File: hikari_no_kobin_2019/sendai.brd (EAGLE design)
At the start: 43 x 43 mm, 4 parts

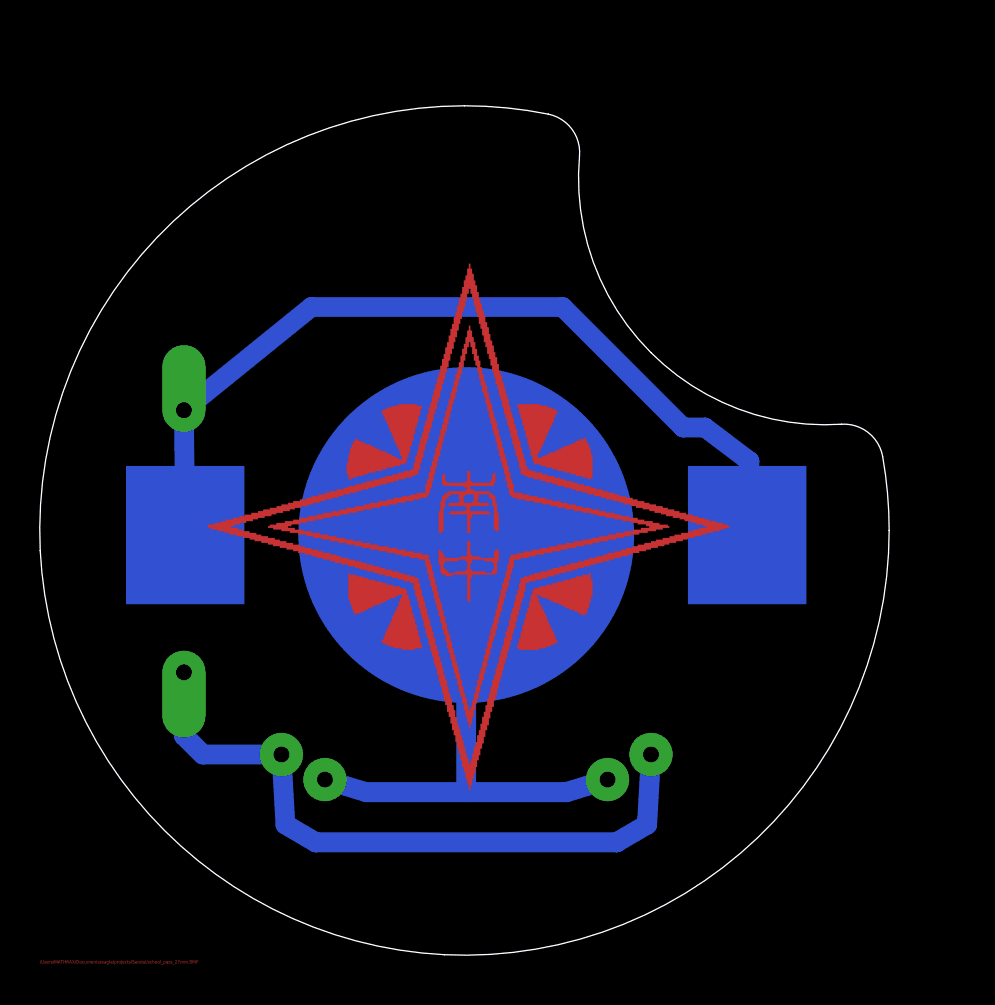
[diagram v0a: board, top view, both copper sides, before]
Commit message: 20190905
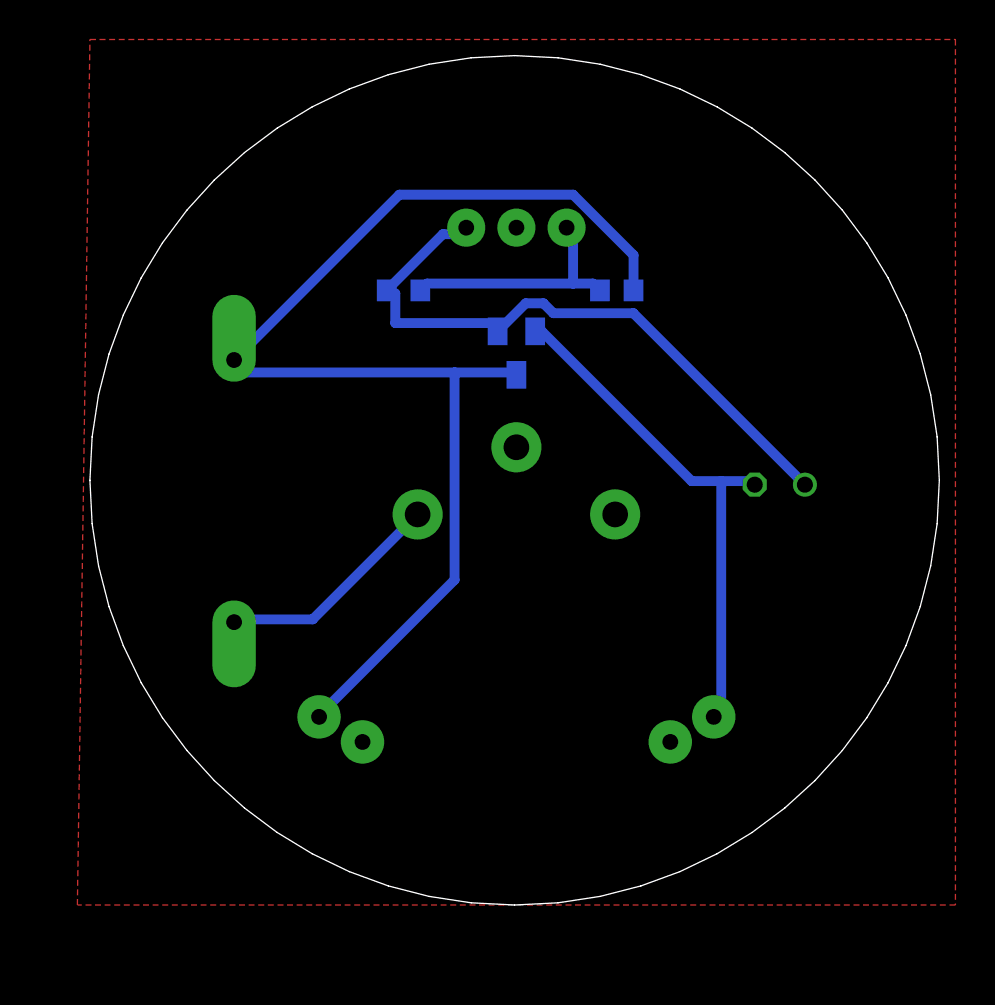
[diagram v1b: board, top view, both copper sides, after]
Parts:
- added C1: 100uF, MATHRAX-a:TT2D6
- added R1: 100, MATHRAX-a:R0603
- added R2: 22k, MATHRAX-a:R0603
- added T1: 2SA1313, DC_LOAD_AU:SOT23-BEC
- added U$5: OSRB38C9AA, sendai:OSRB38C9AA
- U$1: value CR2032_CR2032 -> CR2032_VCR2032_V; device sendai:CR2032_CR2032 -> sendai:CR2032_V
- moved U$3 3.70 mm to (33.0, 11.4)
- moved U$4 3.59 mm to (9.84, 23.5)
- moved U$1 3.59 mm to (24.1, 23.8)
- moved U$2 2.69 mm to (15.2, 11.4)
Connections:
- removed net N$1: U$2.P$1, U$3.P$1, U$4.P$3
- removed net N$2: U$1.-1, U$2.P$2, U$3.P$2
- removed net N$3: U$1.P$1, U$1.P$2, U$4.P$4
- new net 3V: U$1.3, U$4.1
- new net GND: U$1.2, U$2.2, U$3.2, U$5.2
- new net LED1: R1.1, T1.C, U$2.1, U$4.2
- new net LED2: C1.-, T1.E, U$3.1
- new net SENSOR: C1.+, R2.2, T1.B, U$5.1
- new net V: R1.2, R2.1, U$5.3
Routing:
- net LED1: track 0.00 -> 61.6 mm
- net N$3: track 43.6 -> 0.00 mm
- net N$1: track 34.4 -> 0.00 mm
- net SENSOR: track 0.00 -> 32.7 mm
- net N$2: track 27.5 -> 0.00 mm
- net LED2: track 0.00 -> 26.4 mm
- net V: track 0.00 -> 12.3 mm
- net 3V: track 0.00 -> 11.6 mm
- added copper zone on layer 1, net GND
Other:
- outline, holes or cut-outs redrawn
- board text added: "+"
- board text added: "-"
- board text removed: "/Users/MATHRAX/Documents/eagle/projects/Sendai/school_pass_27mm.BMP"
